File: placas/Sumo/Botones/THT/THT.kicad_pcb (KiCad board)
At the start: 2 copper layers, 55.8 x 55.6 mm, 21 parts, among them J1 Conn_02x05_Odd_Even, J2 Screw_Terminal_01x02, SW1 SW_DPDT_x2, SW2 SW_Push, SW3 SW_Push, SW4 SW_Push, SW5 SW_Push

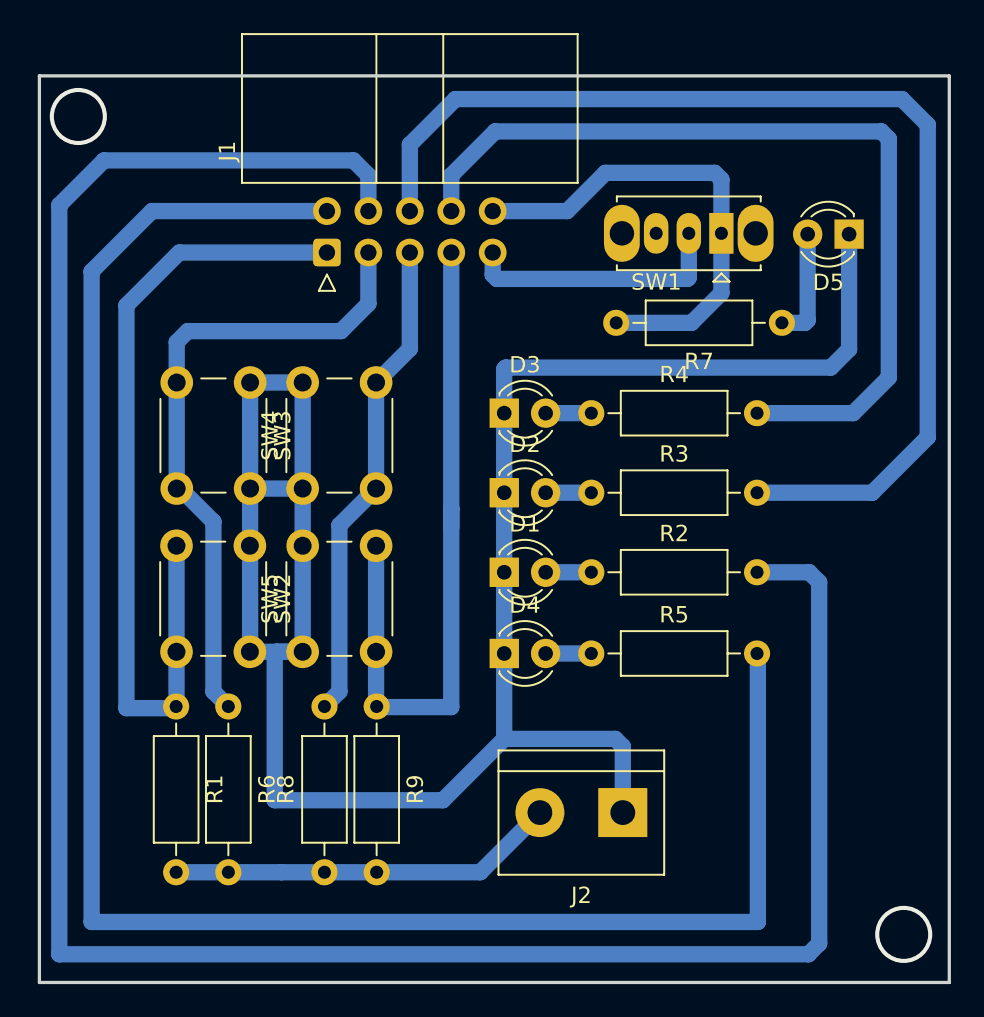
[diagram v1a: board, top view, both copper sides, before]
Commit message: MAI
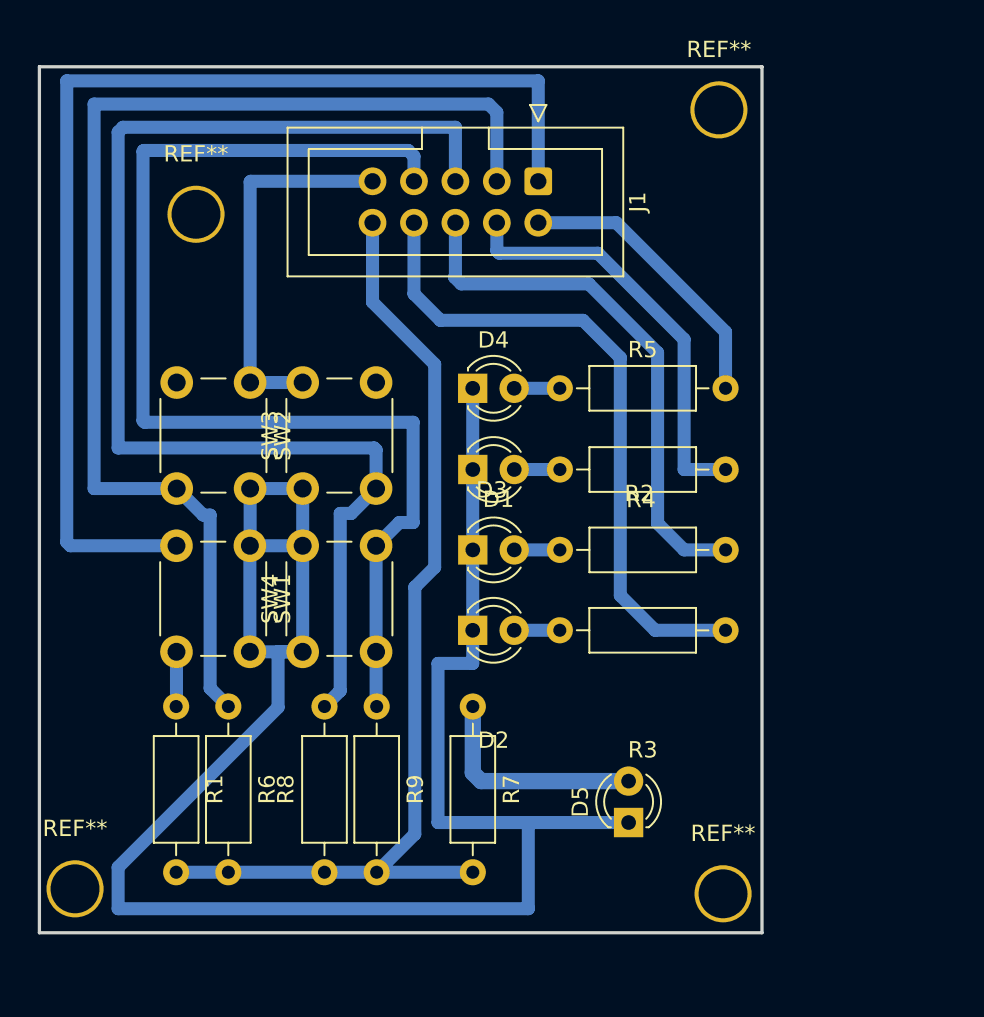
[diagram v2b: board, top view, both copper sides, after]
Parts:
- removed J2: Screw_Terminal_01x02, TerminalBlock:TerminalBlock_bornier-2_P5.08mm
- removed the SW1 at (64.5, 29.5)
- added REF**: MountingHole_2.7mm_Pad, MountingHole:MountingHole_2.7mm_Pad, F.Cu at (32.3, 28.3)
- added REF**: MountingHole_2.7mm_Pad, MountingHole:MountingHole_2.7mm_Pad, F.Cu at (64.6, 70.0)
- added REF**: MountingHole_2.7mm_Pad, MountingHole:MountingHole_2.7mm_Pad, F.Cu at (64.4, 21.9)
- added REF**: MountingHole_2.7mm_Pad, MountingHole:MountingHole_2.7mm_Pad, F.Cu at (24.9, 69.7)
- J1: value Conn_02x05_Odd_Even -> Control Botones; footprint Connector_IDC:IDC-Header_2x05_P2.54mm_Horizontal -> Connector_IDC:IDC-Header_2x05_P2.54mm_Vertical
- moved D5 38.5 mm to (58.8, 65.6), turned to 90 degrees
- moved R7 30.2 mm to (49.3, 58.5), turned to -90 degrees
- moved D4 16.4 mm to (49.3, 39.0)
- moved R5 16.4 mm to (54.6, 39.0)
- moved J1 13.7 mm to (53.3, 26.3), turned to -90 degrees
- moved D3 13.4 mm to (49.3, 53.8)
- moved R4 13.4 mm to (54.6, 53.8)
- moved D1 6.59 mm to (49.3, 44.0)
- moved R2 6.59 mm to (54.6, 44.0)
- moved D2 4.00 mm to (49.3, 48.9)
- moved R3 4.00 mm to (54.6, 48.9)
- renumbered SW2 to SW1, SW3 to SW2, SW4 to SW3, SW5 to SW4
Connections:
- J1 pad 10: /E2 -> /5v
- J1 pad 9: /E1 -> GND
- R7 pad 2: /E2 -> /5v
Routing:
- net /L2: track 141.6 -> 26.0 mm
- net /L1: track 113.2 -> 17.7 mm
- net /B3: track 30.0 -> 76.8 mm
- net /5v: track 23.8 -> 61.1 mm
- net /L3: track 68.7 -> 33.0 mm
- net /B2: track 39.8 -> 72.7 mm
- net /E2: track 29.3 -> 0.00 mm
- net /B4: track 43.6 -> 70.3 mm
- net /B1: track 51.5 -> 73.5 mm
- net /E1: track 16.2 -> 0.00 mm
- net /L4: track 53.9 -> 40.5 mm
- net GND: track 132.1 -> 145.3 mm
- net Net-(D5-Pad2): track 6.92 -> 13.8 mm
- net (no net): vias 2 -> 0
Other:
- board size 55.8 x 55.6 mm -> 44.3 x 53.1 mm
